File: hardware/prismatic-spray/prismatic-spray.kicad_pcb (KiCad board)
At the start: 2 copper layers, 97.5 x 65 mm, 12 parts, among them J2 Conn_01x03_Male, SW1 SW_Push, SW2 SW_Push, SW3 SW_Push, SW4 SW_Push, SW5 RotaryEncoder_Switch, U1 Pico

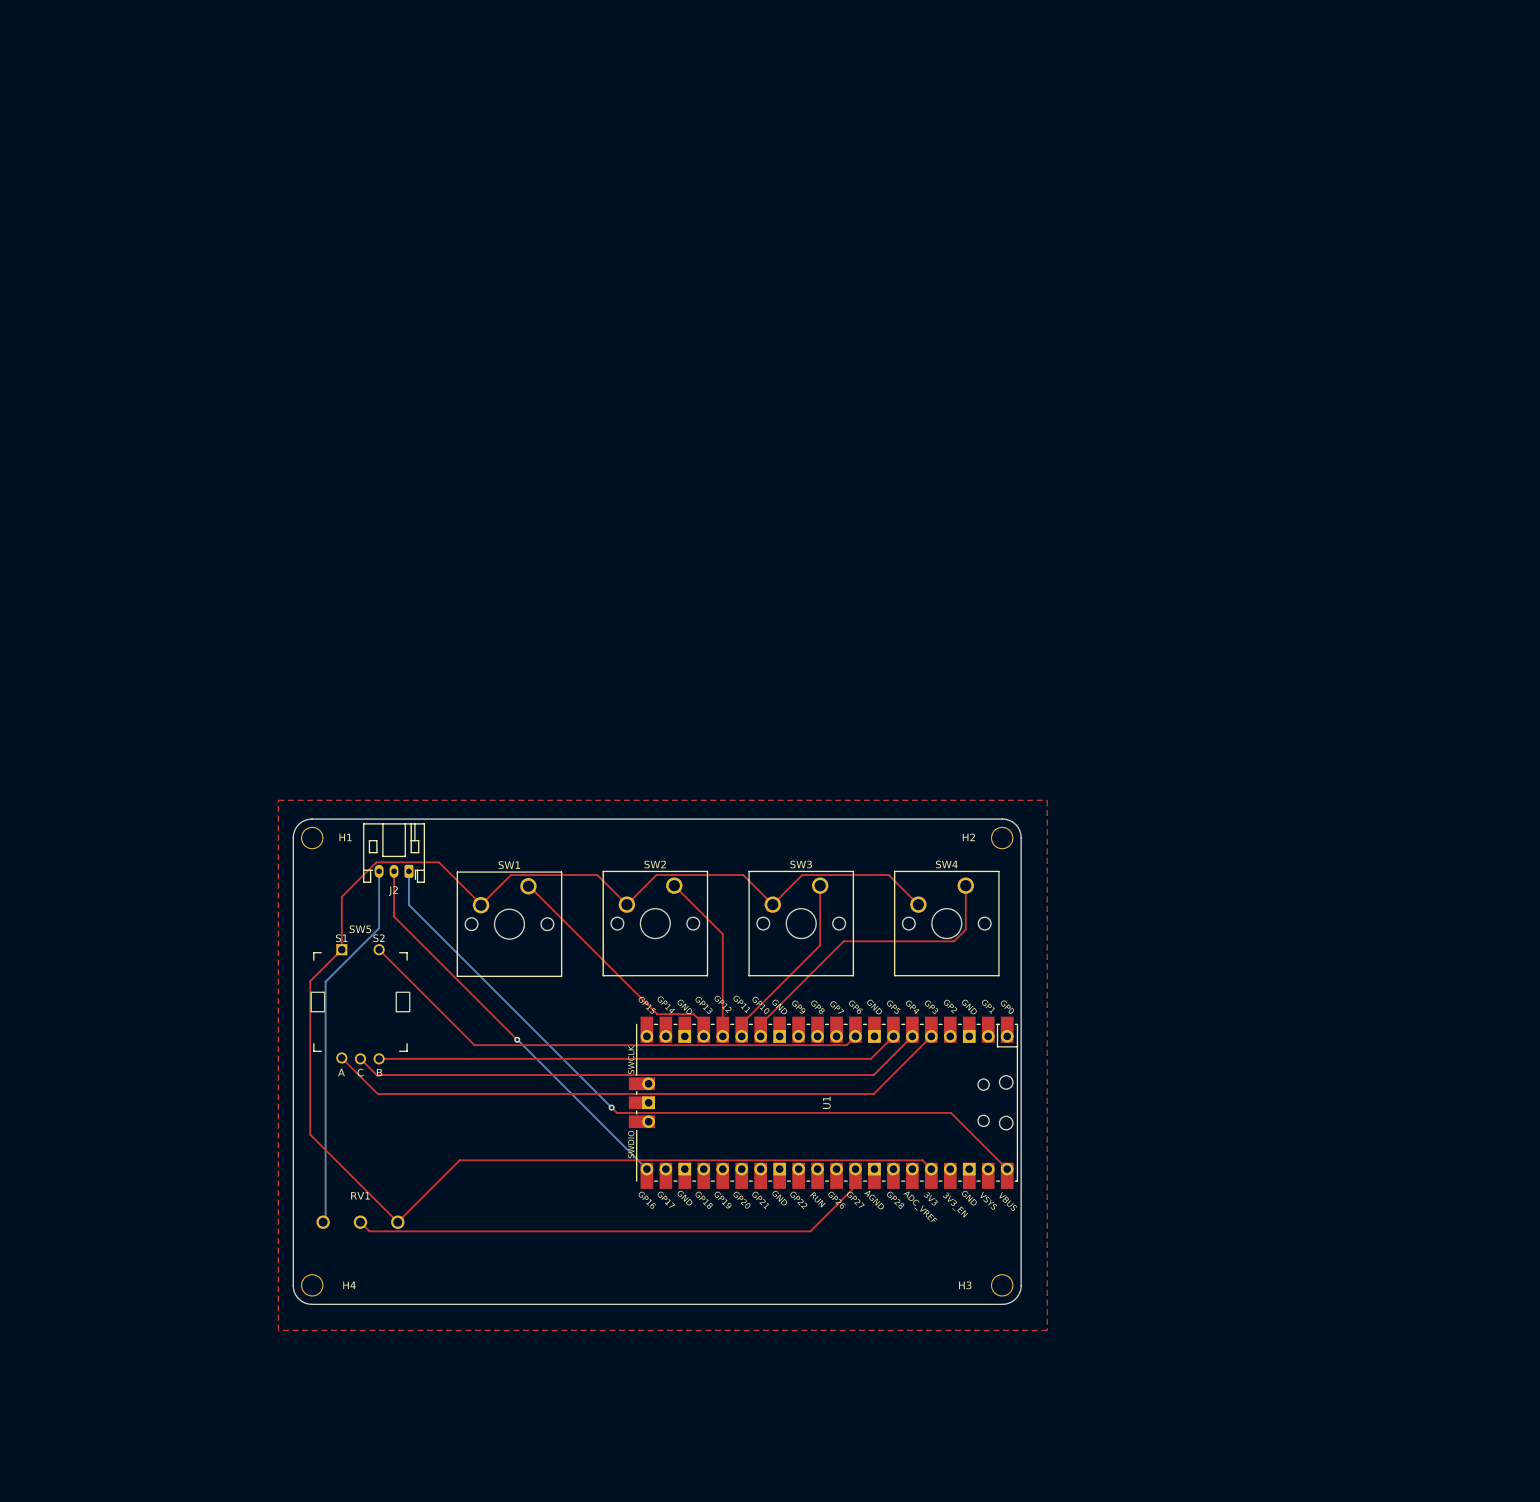
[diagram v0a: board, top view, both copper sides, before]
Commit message: Add rendered image
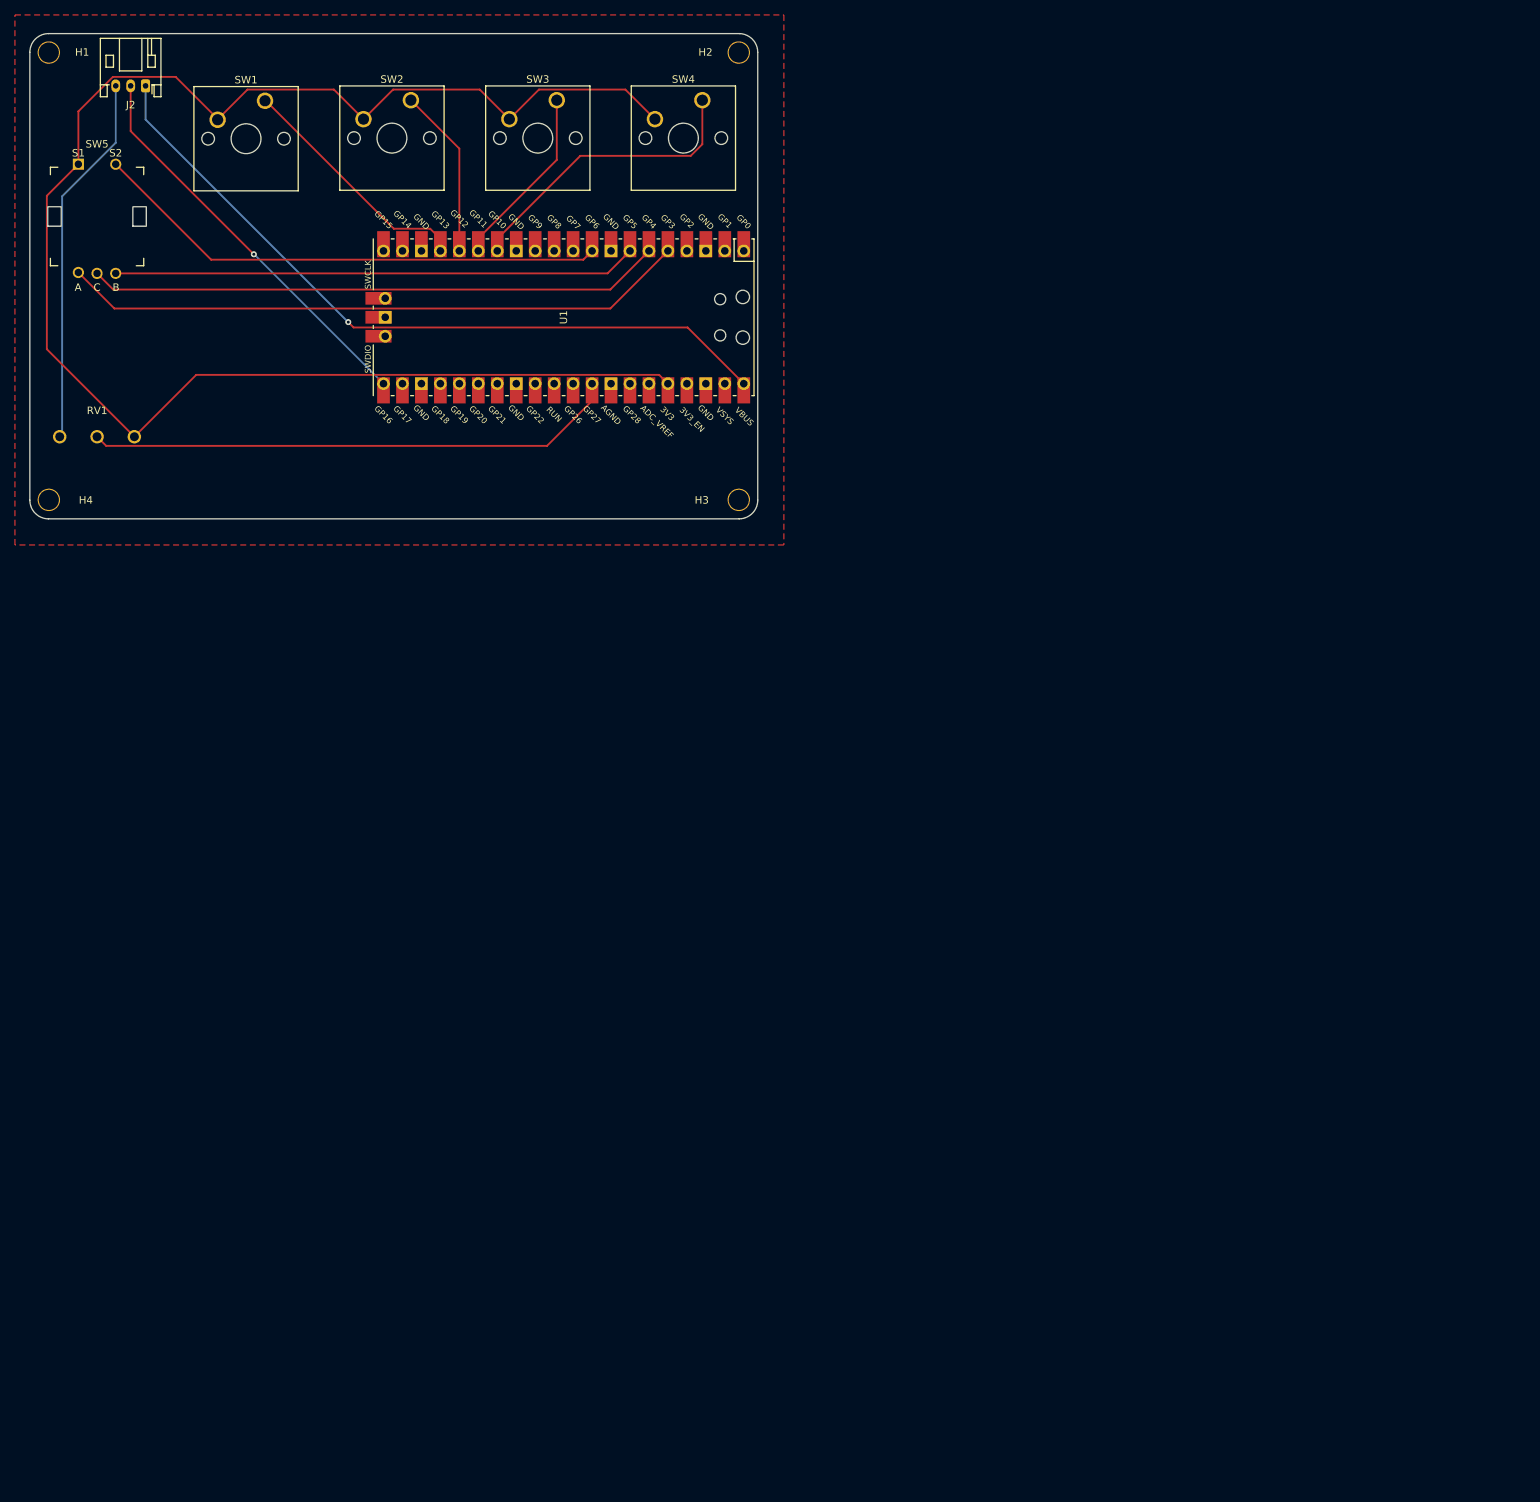
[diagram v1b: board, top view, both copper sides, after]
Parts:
- moved RV1 111.0 mm to (8.72, -10.7)
- moved SW2 111.0 mm to (50.8, -55.8)
- moved SW3 111.0 mm to (70.3, -55.8)
- moved SW4 111.0 mm to (89.8, -55.8)
- moved U1 111.0 mm to (71.2, -26.7)
- moved H1 111.0 mm to (2.26, -62.2)
- moved H2 111.0 mm to (94.7, -62.2)
- moved H3 111.0 mm to (94.7, -2.26)
- moved H4 111.0 mm to (2.26, -2.26)
- moved J2 111.0 mm to (15.2, -57.7)
- moved SW1 111.0 mm to (31.2, -55.7)
- moved SW5 111.0 mm to (8.72, -40.2)

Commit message: finished case
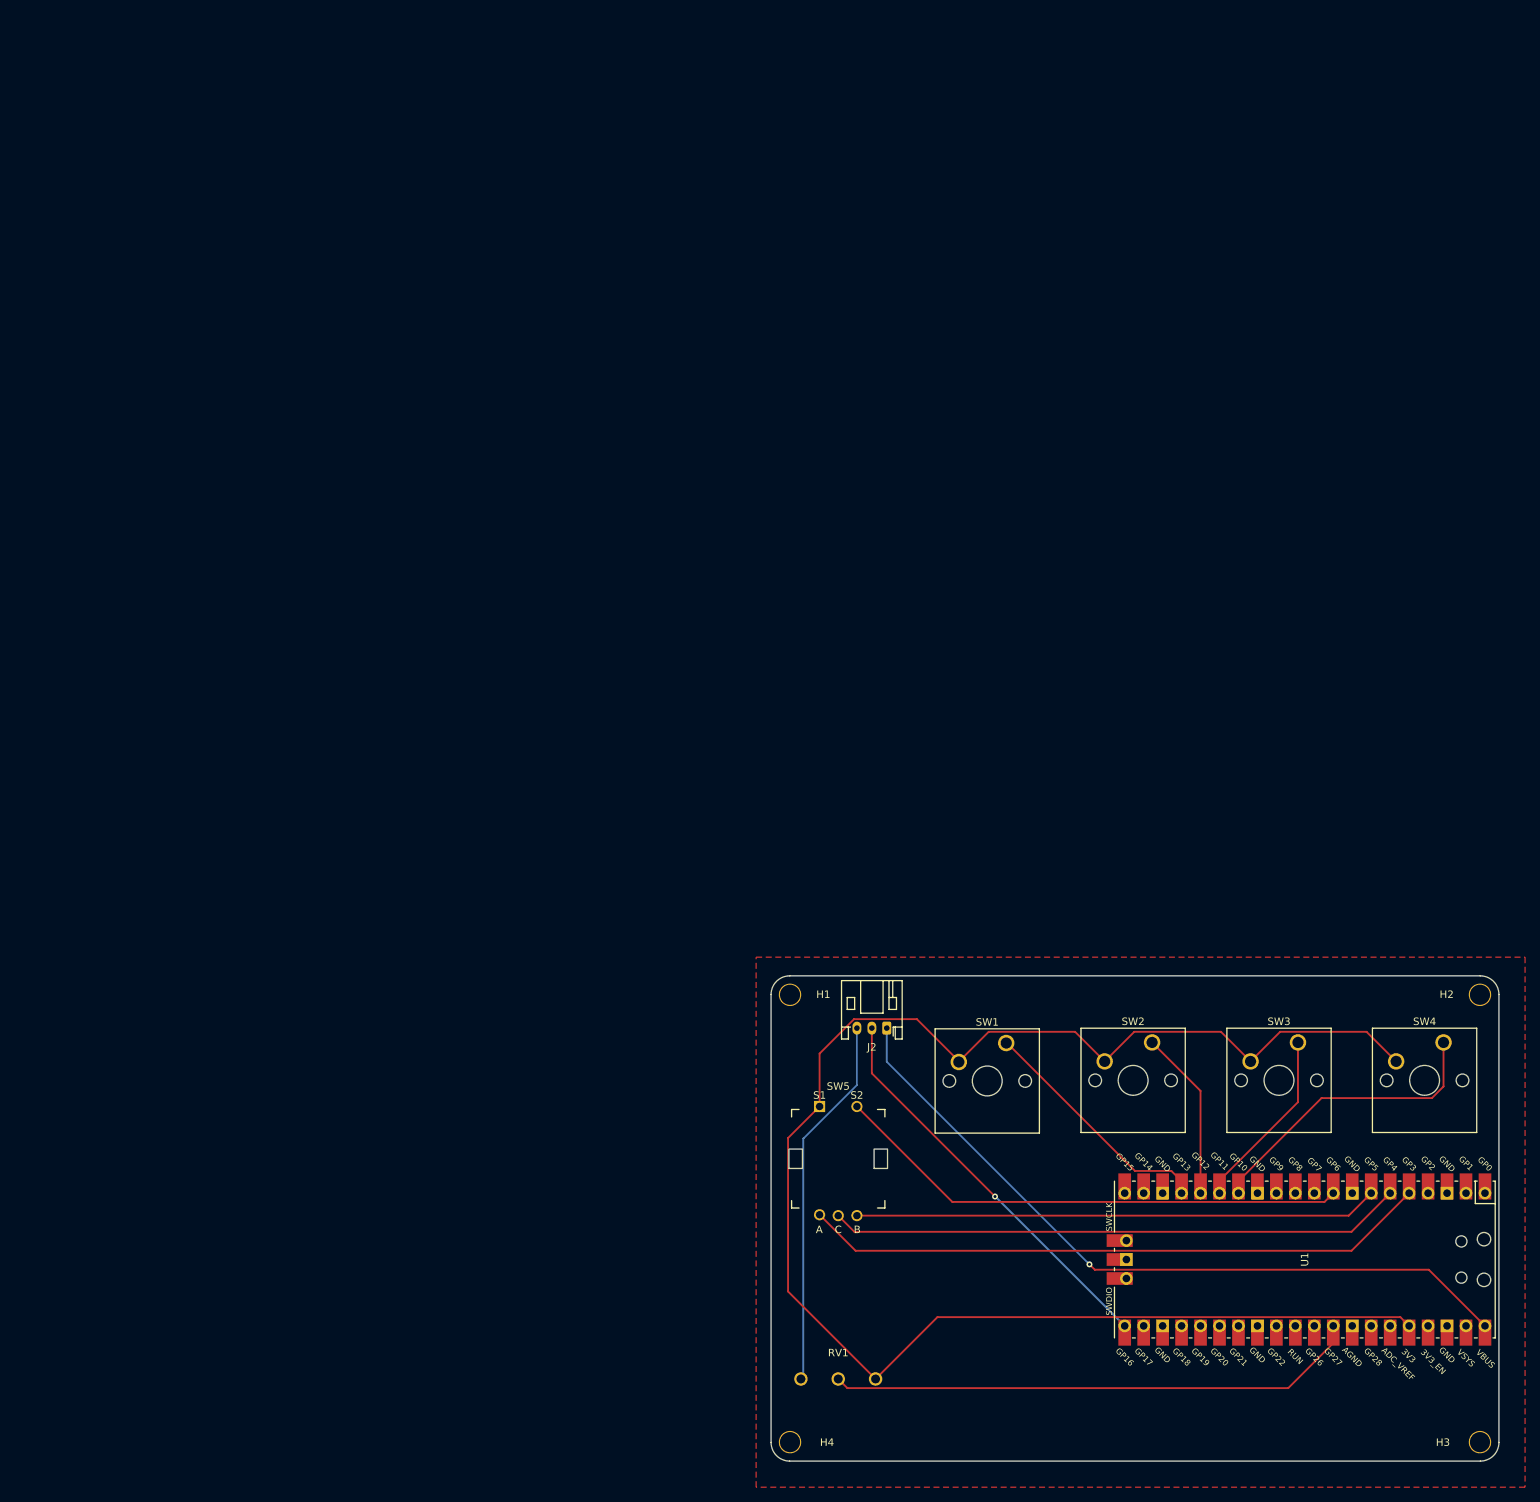
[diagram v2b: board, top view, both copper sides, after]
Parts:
- moved H1 160.6 mm to (101.5, 64.0)
- moved H2 160.6 mm to (194.0, 64.0)
- moved RV1 160.6 mm to (108.0, 115.5)
- moved SW2 160.6 mm to (150.0, 70.4)
- moved SW3 160.6 mm to (169.6, 70.4)
- moved SW4 160.6 mm to (189.1, 70.4)
- moved U1 160.6 mm to (170.5, 99.5)
- moved H3 160.6 mm to (194.0, 124.0)
- moved H4 160.6 mm to (101.5, 124.0)
- moved J2 160.6 mm to (114.5, 68.5)
- moved SW1 160.6 mm to (130.5, 70.5)
- moved SW5 160.6 mm to (108.0, 86.0)
